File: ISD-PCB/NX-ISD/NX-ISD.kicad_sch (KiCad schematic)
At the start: 1 part

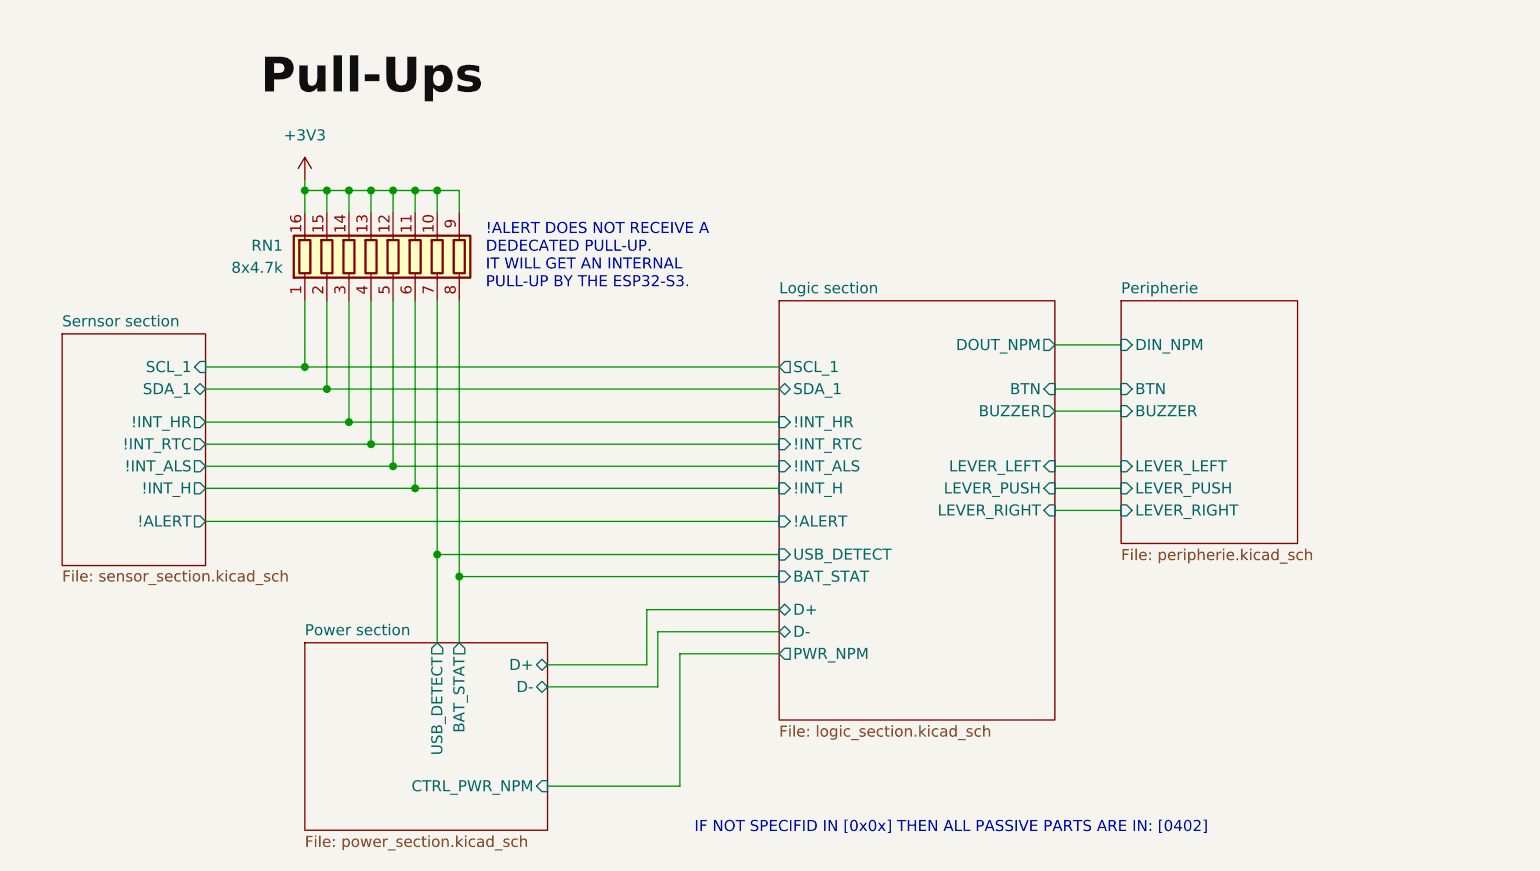
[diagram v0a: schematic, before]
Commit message: v1p1 rework in progress
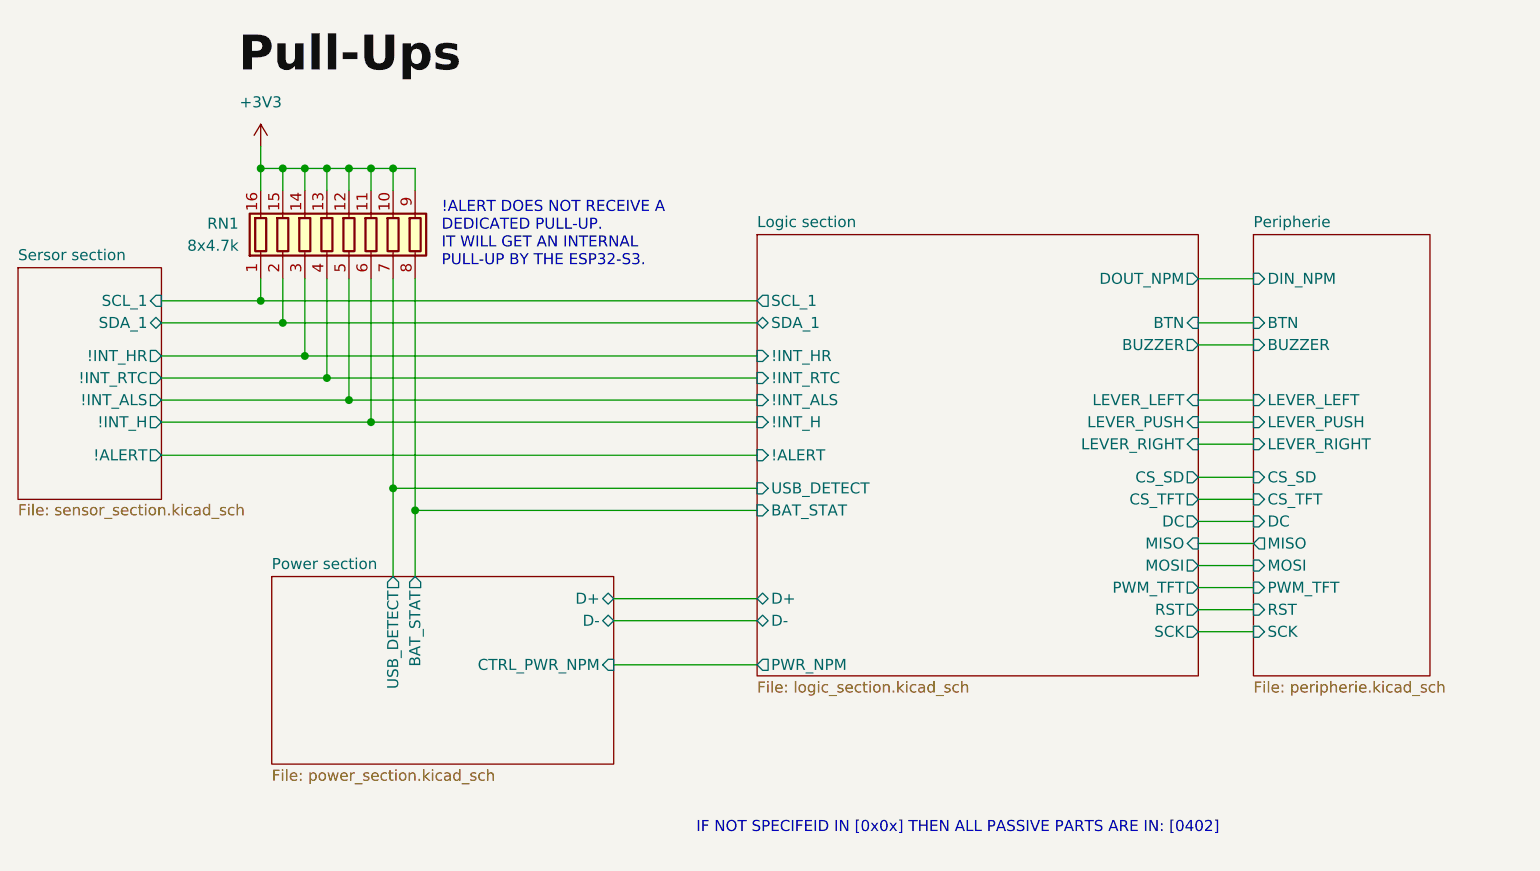
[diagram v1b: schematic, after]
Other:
- sheet Sernsor section renamed Sersor section
- sheet Logic section ports: added CS_SD, CS_TFT, DC, MISO, MOSI, PWM_TFT, RST, SCK; removed none
- sheet Peripherie ports: added CS_SD, CS_TFT, DC, MISO, MOSI, PWM_TFT, RST, SCK; removed none
- note added: "!ALERT DOES NOT RECEIVE A DEDICATED PULL-UP. IT WILL GET AN INTERNAL PULL-UP BY THE ESP32-S3."
- note added: "IF NOT SPECIFEID IN [0x0x] THEN ALL PASSIVE PARTS ARE IN: [0402]"
- note removed: "!ALERT DOES NOT RECEIVE A DEDECATED PULL-UP. IT WILL GET AN INTERNAL PULL-UP BY THE ESP32-S3."
- note removed: "IF NOT SPECIFID IN [0x0x] THEN ALL PASSIVE PARTS ARE IN: [0402]"
- moved on the sheet: RN1
